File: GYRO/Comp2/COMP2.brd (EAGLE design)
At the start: 29.2 x 16.2 mm, 15 parts, among them U2 LSM9DS0TR

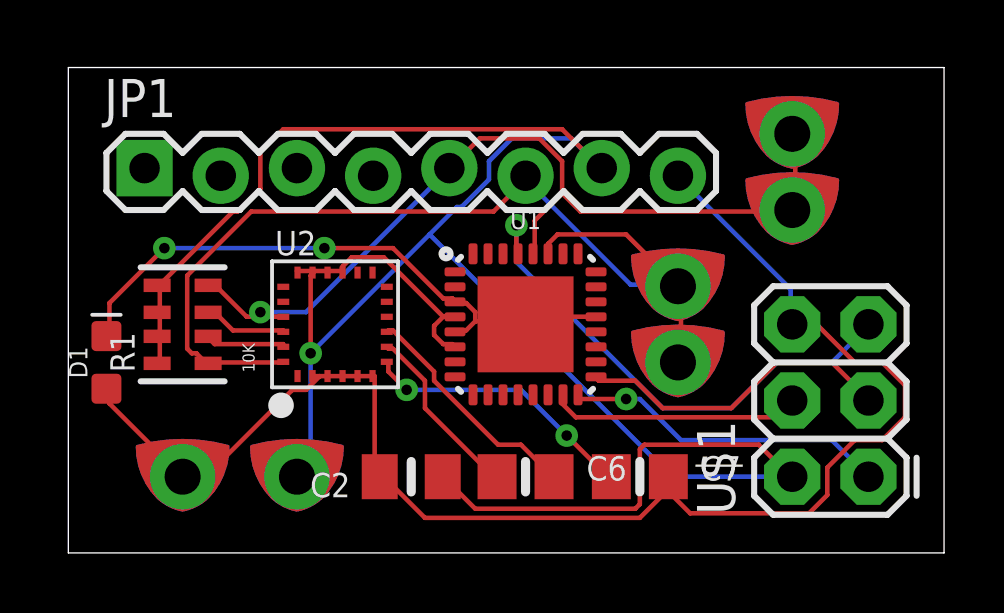
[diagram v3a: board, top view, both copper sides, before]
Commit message: S
S
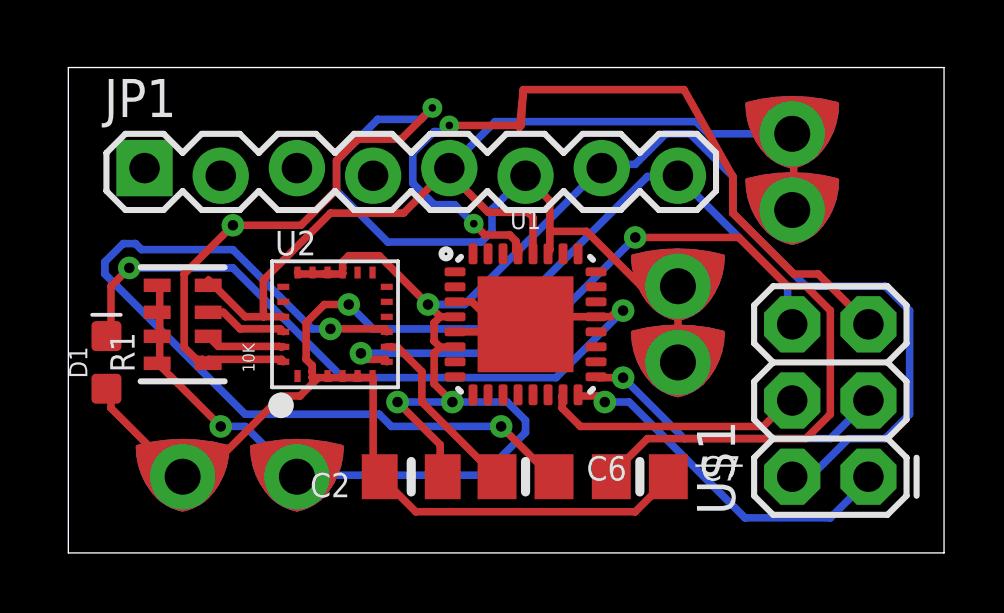
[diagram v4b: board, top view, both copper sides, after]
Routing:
- net N$6: track 9.25 -> 30.9 mm
- net N$2: track 7.79 -> 29.1 mm, vias 0 -> 2
- net VCC: track 79.6 -> 65.6 mm, vias 1 -> 4
- net RESET: track 17.1 -> 28.3 mm, vias 1 -> 2
- net N$4: track 20.3 -> 29.4 mm
- net SDA: track 33.5 -> 41.1 mm, vias 0 -> 2
- net SCL: track 30.0 -> 31.7 mm, vias 1 -> 0
- net MISO: track 10.8 -> 12.0 mm
- net GND: track 49.3 -> 49.8 mm, vias 0 -> 1
- net SCK: track 10.7 -> 10.5 mm, vias 0 -> 1
